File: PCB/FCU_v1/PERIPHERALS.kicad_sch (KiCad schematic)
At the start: 63 parts, among them J11 USB_C_Receptacle_USB2.0_16P, J4 Conn_Coaxial_Small, U10 SN65HVD232, U3 TLV75533PDYDR, U4 BMI088, U5 LIS2MDL, U6 LPS22HH, U7 W25Q64JV, U8 USBLC6-2SC6, U9 MAX-M10M-20B

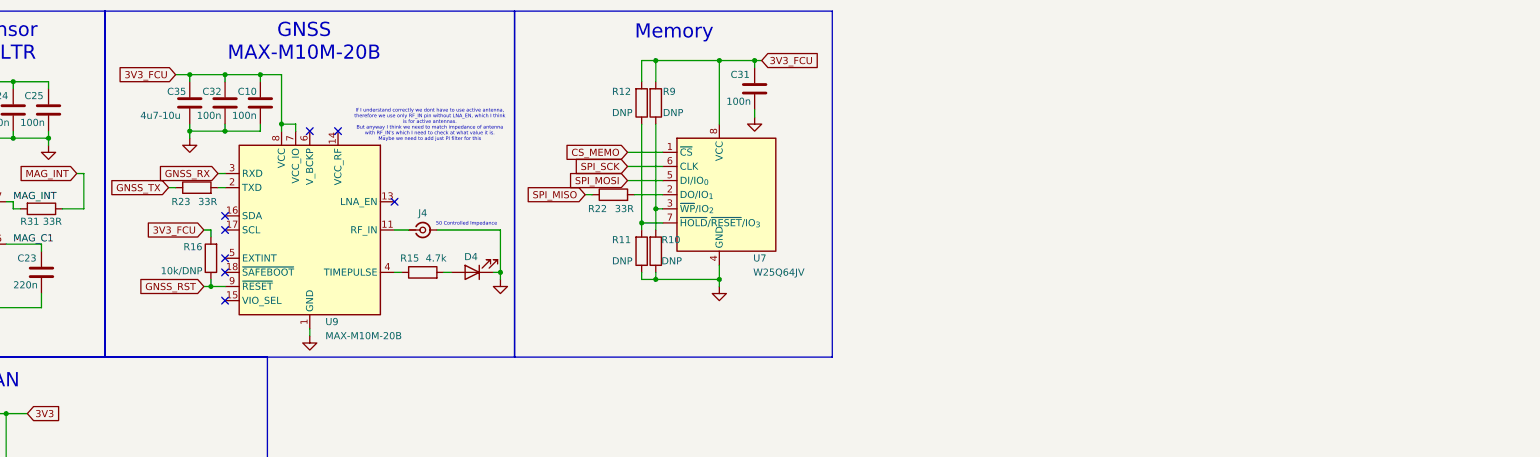
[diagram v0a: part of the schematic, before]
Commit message: Layout update
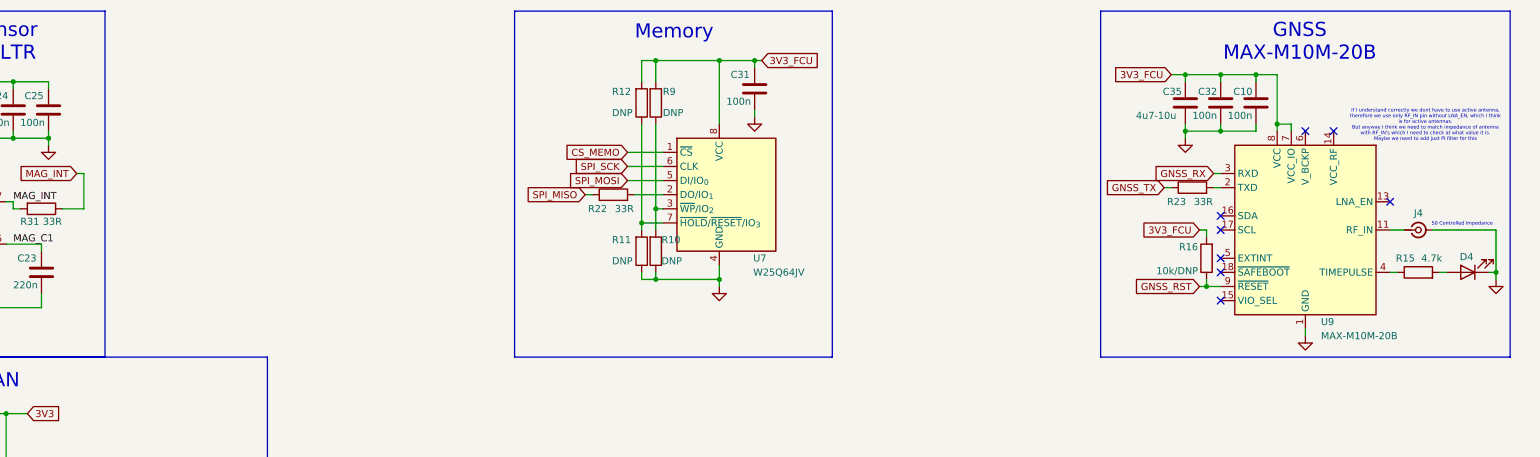
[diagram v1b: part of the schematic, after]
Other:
- moved on the sheet: C10, C32, C35, D4, J4, R15, R16, R23, U9
